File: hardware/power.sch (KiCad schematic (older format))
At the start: 69 parts, among them P1 CONN_01X02_CBAT, P2 CONN_01X02_FAN, Q1 DMG4712SSS, Q2 DMG4712SSS, U10 MCP1501T-30E, U11 PDM1-S, U12 MIC5225-5.0, U21 74LVC1G17, U7 MIC5225-5.0, U8 LT3471, U9 R-78E3.3-0.5

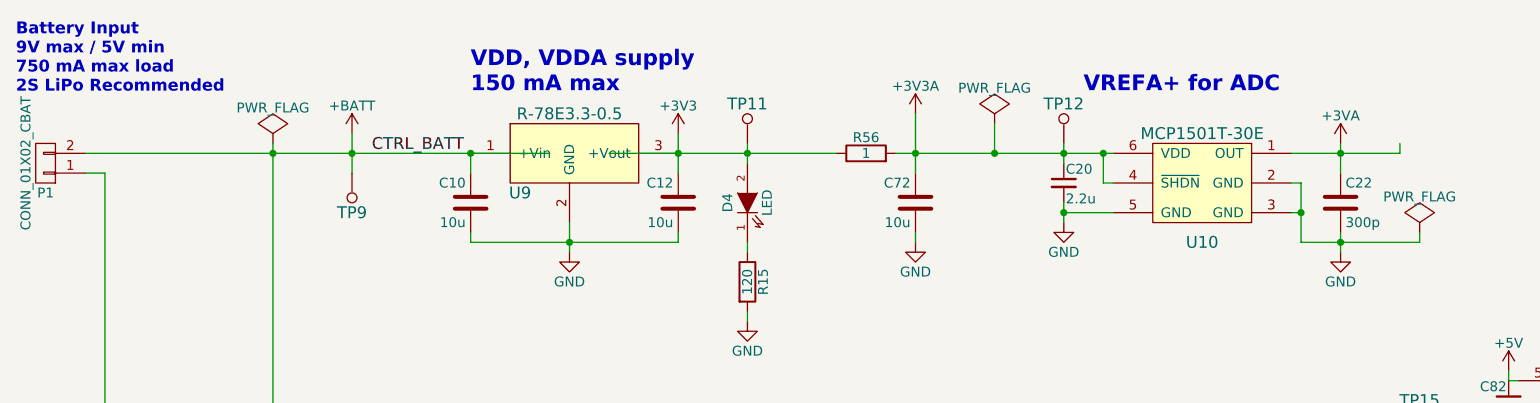
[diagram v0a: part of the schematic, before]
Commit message: tweaks, testpoints, decluttering
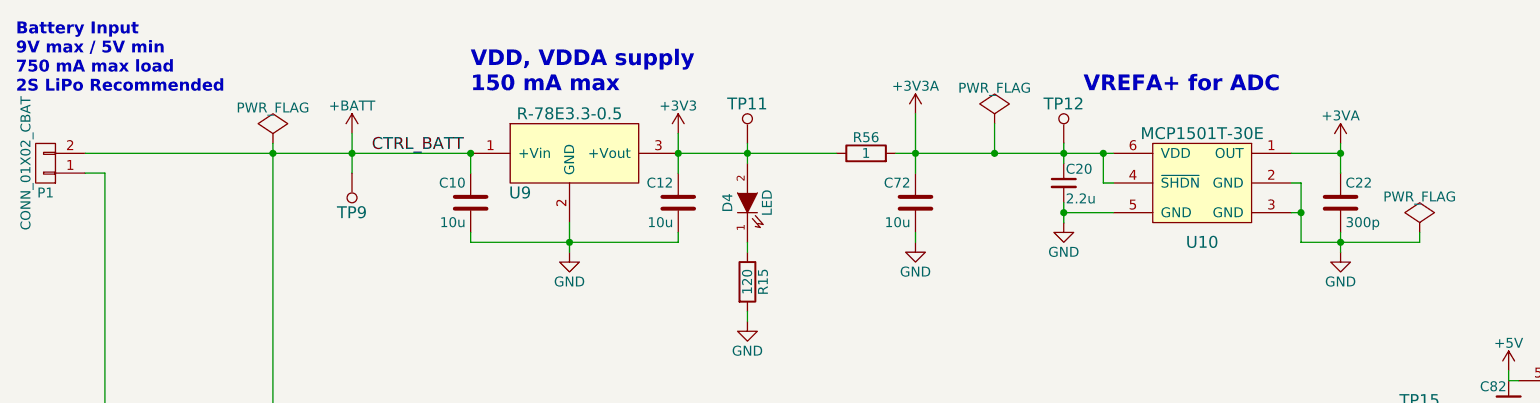
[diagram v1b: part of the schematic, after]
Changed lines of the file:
@@
 FAN_DRAIN
-Wire Wire Line
-	1150 1150 3500 1150
 Wire Wire Line
 	1150 1250 1250 1250
@@
 	10250 4300 10250 4250
 Wire Wire Line
-	7250 1150 7800 1150
-Wire Wire Line
 	7250 1450 7300 1450
 Wire Wire Line
@@
 Connection ~ 6100 1150
 Wire Wire Line
-	7500 1100 7500 1250
-Connection ~ 7500 1150
-Wire Wire Line
 	7500 1550 7500 1650
 Wire Wire Line
@@
 	4150 1050 4150 1250
 Connection ~ 3600 1600
-Wire Wire Line
-	3800 1150 4950 1150
 Wire Wire Line
 	5250 1150 6350 1150
@@
 Connection ~ 5200 5800
 Wire Wire Line
-	3100 1250 3100 1150
+	3100 1150 3100 1250
 Wire Wire Line
 	4150 1600 4150 1550
@@
 Wire Wire Line
 	8350 3050 8350 3100
-Wire Wire Line
-	7800 1150 7800 1100
 Wire Wire Line
 	7900 2600 7900 2700
@@
 Wire Wire Line
 	2600 7250 2600 7300
+Wire Wire Line
+	4150 1150 4950 1150
+Wire Wire Line
+	1150 1150 3100 1150
+Wire Wire Line
+	7500 1250 7500 1100
+Wire Wire Line
+	7250 1150 7500 1150
+Connection ~ 7500 1150
 $EndSCHEMATC
